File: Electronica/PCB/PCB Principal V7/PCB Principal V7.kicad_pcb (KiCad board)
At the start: 2 copper layers, 151.8 x 74 mm, 21 parts, among them J1 Conexion Sensores, J11 Conn_01x04_Pin, J2 Power Monster, J3 On/Off General, J4 Power Input 2, J5 IDC Placa Botones, J6 Power Input 1, SW1 On/Off Motores, U1 74HC595

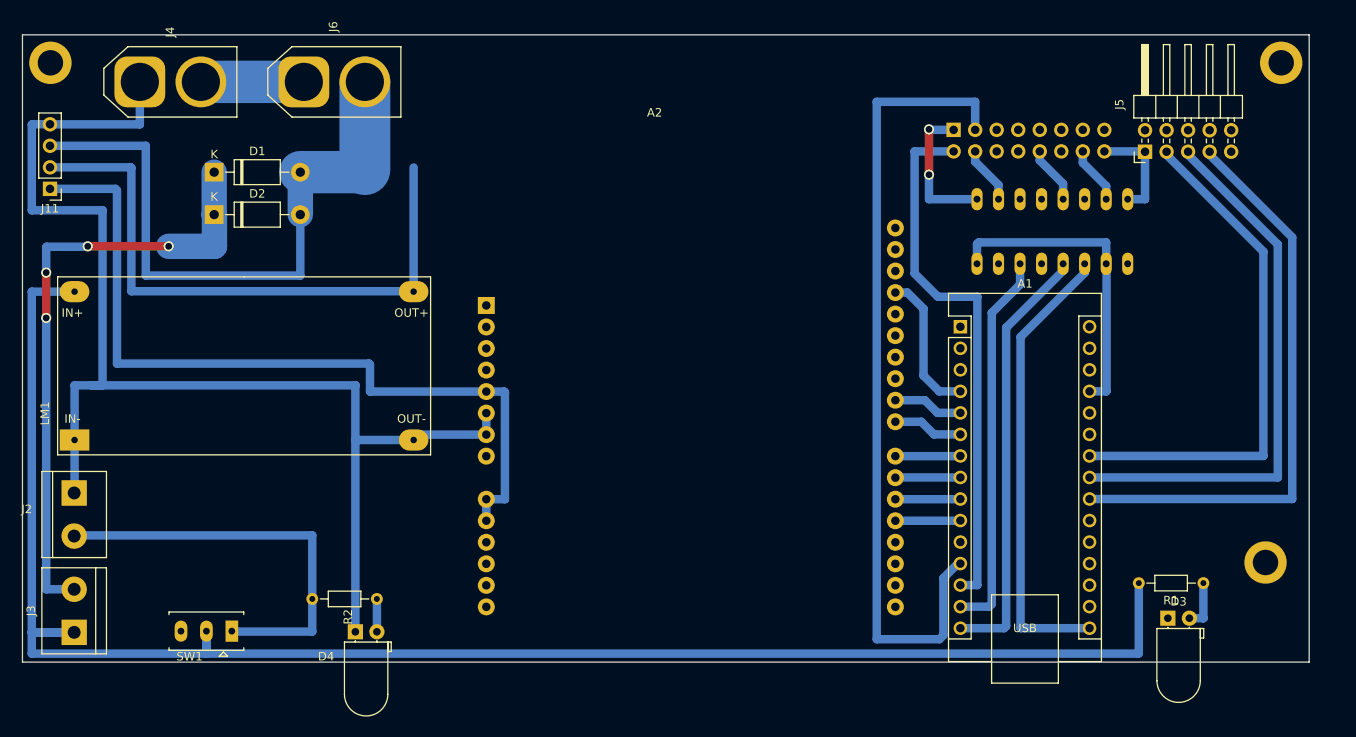
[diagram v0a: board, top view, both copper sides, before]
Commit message: PCB sensores v2 y principal v7 terminadas
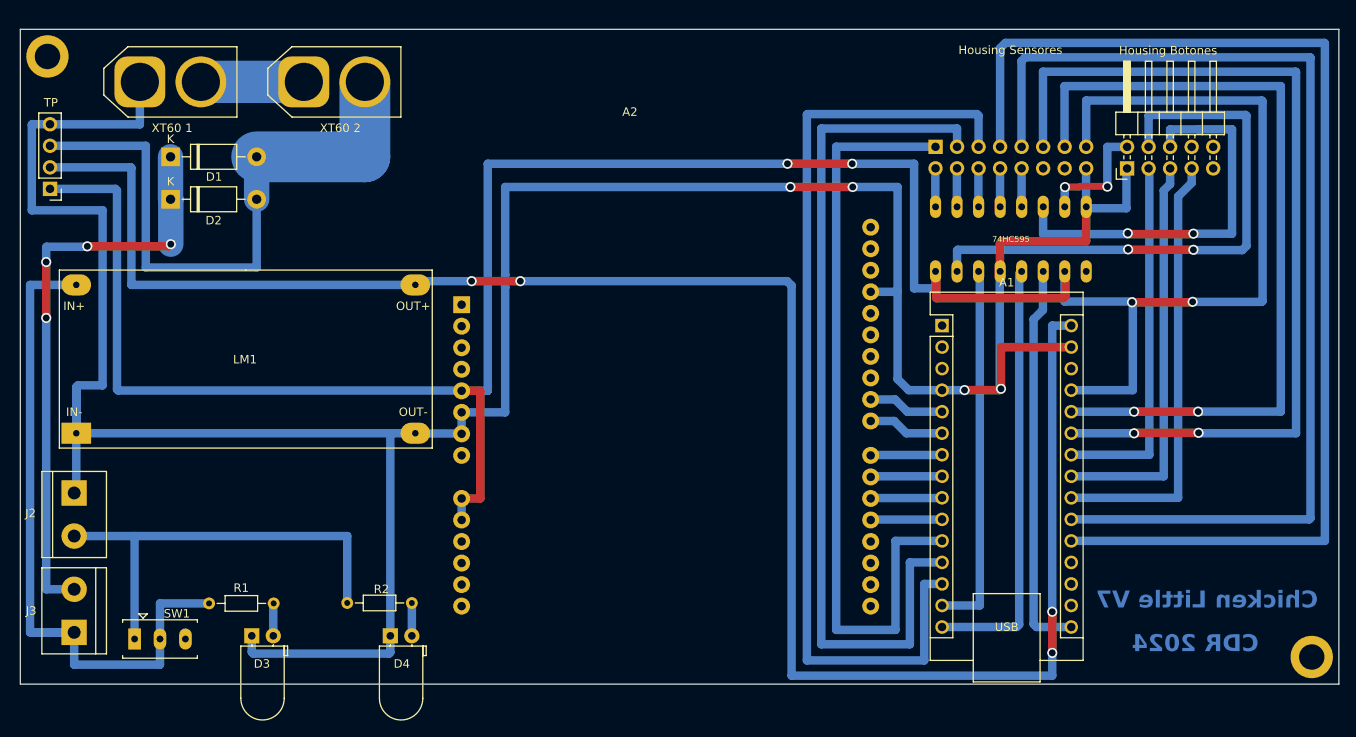
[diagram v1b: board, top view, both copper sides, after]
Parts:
- removed the ? at (226.4, 47.5)
- Housing Botones: renamed from J5
- Housing Sensores: renamed from J1
- XT60 1: renamed from J4
- XT60 2: renamed from J6
- moved R1 109.7 mm to (99.9, 111.3)
- moved D3 108.1 mm to (105.0, 115.2)
- moved ? 12.4 mm to (230.0, 117.7)
- moved SW1 9.52 mm to (92.1, 115.5), turned to 0 degrees
- moved D1 5.46 mm to (95.4, 58.6)
- moved D2 5.46 mm to (95.4, 63.6)
- moved 74HC595 4.97 mm to (194.5, 68.3)
- moved D4 4.15 mm to (121.3, 115.2)
- moved R2 4.15 mm to (116.2, 111.3)
- moved Housing Sensores 2.93 mm to (185.6, 57.5)
- moved A2 2.91 mm to (129.7, 76.1)
- moved Housing Botones 2.89 mm to (208.2, 60.0)
- moved A1 2.16 mm to (186.4, 78.5)
- moved ? 0.83 mm to (80.8, 46.8)
- moved LM1 0.82 mm to (104.2, 82.5)
- renumbered U1 to 74HC595, J11 to TP
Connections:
- 74HC595 pad 4: LED2 -> TRIG 4
- 74HC595 pad 5: TRIG 4 -> TRIG 1
- 74HC595 pad 7: TRIG 1 -> LED2
- A1 pad 25: CNY 1 -> CNY 2
- A1 pad 26: CNY 2 -> CNY 1
- Housing Sensores pad 1: TRIG 2 -> ECHO 1
- Housing Sensores pad 10: TRIG 4 -> TRIG 1
- Housing Sensores pad 12: ECHO 1 -> unconnected-(J1-Pin_12-Pad12)
- Housing Sensores pad 13: CNY 3 -> CNY 1
- Housing Sensores pad 14: TRIG 1 -> unconnected-(J1-Pin_14-Pad14)
- Housing Sensores pad 2: ECHO 3 -> TRIG 2
- Housing Sensores pad 5: TRIG 5 -> ECHO 3
- Housing Sensores pad 6: unconnected-(J1-Pin_6-Pad6) -> TRIG 5
- Housing Sensores pad 7: ECHO 5 -> ECHO 4
- Housing Sensores pad 8: ECHO 4 -> TRIG 4
- Housing Sensores pad 9: CNY 1 -> ECHO 5
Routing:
- net +5V: track 132.0 -> 307.3 mm, vias 0 -> 4
- net GND: track 181.0 -> 344.9 mm, vias 0 -> 4
- net VNano: track 72.1 -> 222.9 mm, vias 0 -> 4
- net ECHO 4: track 0.00 -> 138.9 mm
- net ECHO 5: track 0.00 -> 127.0 mm
- net MOTORES: track 201.1 -> 83.6 mm
- net CNY 2: track 0.00 -> 107.9 mm, vias 0 -> 2
- net CNY 1: track 0.00 -> 95.8 mm, vias 0 -> 2
- net ECHO 1: track 0.00 -> 91.7 mm
- net LED3: track 0.00 -> 67.6 mm, vias 0 -> 2
- net ECHO 3: track 63.6 -> 113.4 mm
- net LED4: track 0.00 -> 47.3 mm, vias 0 -> 2
- net BTN2: track 61.1 -> 43.0 mm
- net BTN1: track 65.0 -> 47.5 mm
- net LED1: track 68.9 -> 52.1 mm
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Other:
- board size 151.8 x 74 mm -> 155.5 x 77.2 mm
- board text added: "CDR 2024"
- board text added: "Chicken Little V7"
